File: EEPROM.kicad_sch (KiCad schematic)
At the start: 22 parts, among them IC1 PCA6408A_TSSOP, IC2 AT24CS01_SOT23, U2 TPS613221A_SOT-23-5

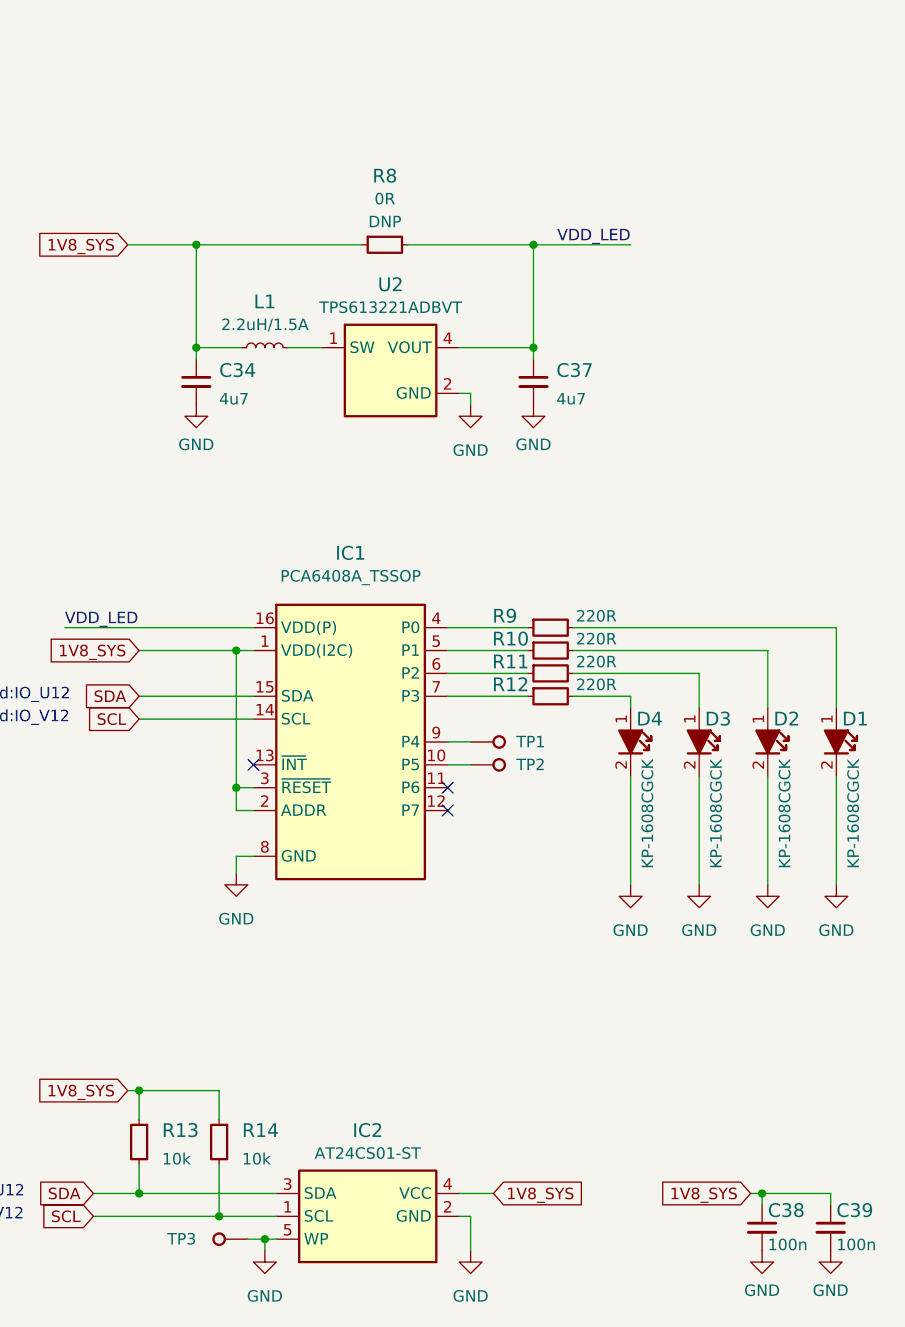
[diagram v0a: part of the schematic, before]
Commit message: Update designators
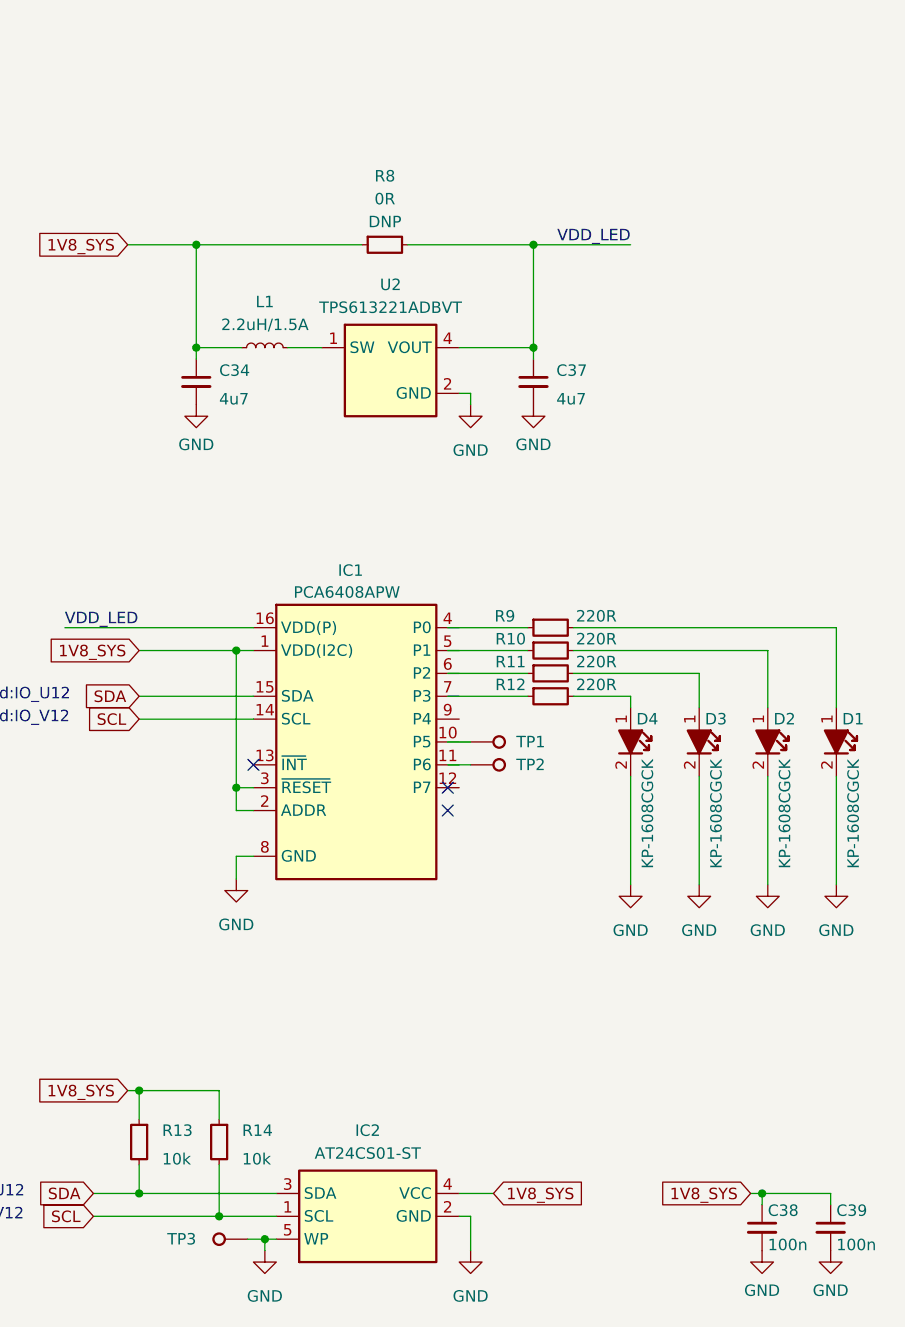
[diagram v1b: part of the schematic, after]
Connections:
- net at R9.1: no longer IC1.4 (P0)
- net at R10.1: no longer IC1.5 (P1)
- net at R11.1: no longer IC1.6 (P2)
- net at R12.1: no longer IC1.7 (P3)
- net at TP2.1: no longer IC1.10 (P5)
- net at TP1.1: no longer IC1.9 (P4)
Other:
- moved on the sheet: IC1
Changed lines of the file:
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@@
     (stroke (width 0) (type default))
   )
-  (wire (pts (xy 193.675 138.43) (xy 193.675 136.525))
+  (wire (pts (xy 193.675 139.065) (xy 193.675 136.525))
     (stroke (width 0) (type default))
   )
@@
     (in_bom yes) (on_board yes) (dnp no) (fields_autoplaced)
     (property "Reference" "C34" (at 191.77 82.5563 90)
-      (effects (font (size 1.524 1.524)) (justify left))
+      (effects (font (size 1.27 1.27)) (justify left))
     )
     (property "Value" "C_4u7_0402" (at 179.07 101.6 0)
@@
     (in_bom yes) (on_board yes) (dnp no) (fields_autoplaced)
     (property "Reference" "C37" (at 229.235 82.5563 90)
-      (effects (font (size 1.524 1.524)) (justify left))
+      (effects (font (size 1.27 1.27)) (justify left))
     )
     (property "Value" "C_4u7_0402" (at 216.535 101.6 0)
@@
     (in_bom yes) (on_board yes) (dnp no)
     (property "Reference" "IC2" (at 208.28 167.005 0)
-      (effects (font (size 1.524 1.524)))
+      (effects (font (size 1.27 1.27)))
     )
     (property "Value" "AT24CS01_SOT23" (at 208.28 168.91 0)
@@
     (in_bom yes) (on_board yes) (dnp no)
     (property "Reference" "R8" (at 210.185 60.96 0)
-      (effects (font (size 1.524 1.524)))
+      (effects (font (size 1.27 1.27)))
     )
     (property "Value" "R_0R_0402" (at 227.965 81.28 0)
@@
     (in_bom yes) (on_board yes) (dnp no) (fields_autoplaced)
     (property "Reference" "R13" (at 185.42 167.005 90)
-      (effects (font (size 1.524 1.524)) (justify left))
+      (effects (font (size 1.27 1.27)) (justify left))
     )
     (property "Value" "R_10k_0402" (at 170.18 186.055 0)
@@
     (in_bom yes) (on_board yes) (dnp no)
     (property "Reference" "R9" (at 223.52 109.855 0)
-      (effects (font (size 1.524 1.524)))
+      (effects (font (size 1.27 1.27)))
     )
     (property "Value" "R_220R_0402" (at 246.38 123.825 0)
@@
     (in_bom yes) (on_board yes) (dnp no)
     (property "Reference" "R10" (at 224.155 112.395 0)
-      (effects (font (size 1.524 1.524)))
+      (effects (font (size 1.27 1.27)))
     )
     (property "Value" "R_220R_0402" (at 246.38 126.365 0)
@@
     (in_bom yes) (on_board yes) (dnp no)
     (property "Reference" "R11" (at 224.155 114.935 0)
-      (effects (font (size 1.524 1.524)))
+      (effects (font (size 1.27 1.27)))
     )
     (property "Value" "R_220R_0402" (at 246.38 128.905 0)
@@
     (in_bom yes) (on_board yes) (dnp no)
     (property "Reference" "D4" (at 238.125 121.285 90)
-      (effects (font (size 1.524 1.524)) (justify left))
+      (effects (font (size 1.27 1.27)) (justify left))
     )
     (property "Value" "LED_G_0603_KP-1608CGCK" (at 241.3 125.7299 90)
@@
     (in_bom yes) (on_board yes) (dnp no)
     (property "Reference" "R12" (at 224.155 117.475 0)
-      (effects (font (size 1.524 1.524)))
+      (effects (font (size 1.27 1.27)))
     )
     (property "Value" "R_220R_0402" (at 246.38 131.445 0)
@@
     (in_bom yes) (on_board yes) (dnp no)
     (property "Reference" "C38" (at 252.73 175.895 90)
-      (effects (font (size 1.524 1.524)) (justify left))
+      (effects (font (size 1.27 1.27)) (justify left))
     )
     (property "Value" "C_100n_0402" (at 241.935 195.58 0)
@@
     (in_bom yes) (on_board yes) (dnp no)
     (property "Reference" "D3" (at 245.745 121.285 90)
-      (effects (font (size 1.524 1.524)) (justify left))
+      (effects (font (size 1.27 1.27)) (justify left))
     )
     (property "Value" "LED_G_0603_KP-1608CGCK" (at 248.92 125.7299 90)
@@
     (in_bom yes) (on_board yes) (dnp no)
     (property "Reference" "D2" (at 253.365 121.285 90)
-      (effects (font (size 1.524 1.524)) (justify left))
+      (effects (font (size 1.27 1.27)) (justify left))
     )
     (property "Value" "LED_G_0603_KP-1608CGCK" (at 256.54 125.7299 90)
@@
     (in_bom yes) (on_board yes) (dnp no)
     (property "Reference" "D1" (at 260.985 121.285 90)
-      (effects (font (size 1.524 1.524)) (justify left))
+      (effects (font (size 1.27 1.27)) (justify left))
     )
     (property "Value" "LED_G_0603_KP-1608CGCK" (at 264.16 125.7299 90)
@@
     )
   )
-  (symbol (lib_id "antmicropower:GND") (at 193.675 138.43 0) (unit 1)
+  (symbol (lib_id "antmicropower:GND") (at 193.675 139.065 0) (unit 1)
     (in_bom yes) (on_board yes) (dnp no) (fields_autoplaced)
-    (property "Reference" "#PWR0113" (at 193.675 144.78 0)
+    (property "Reference" "#PWR0113" (at 193.675 145.415 0)
       (effects (font (size 1.27 1.27)) hide)
     )
-    (property "Value" "GND" (at 193.675 143.51 0)
+    (property "Value" "GND" (at 193.675 144.145 0)
       (effects (font (size 1.27 1.27)))
     )
-    (property "Footprint" "" (at 193.675 138.43 0)
+    (property "Footprint" "" (at 193.675 139.065 0)
       (effects (font (size 1.27 1.27)) hide)
     )
-    (property "Datasheet" "" (at 193.675 138.43 0)
+    (property "Datasheet" "" (at 193.675 139.065 0)
       (effects (font (size 1.27 1.27)) hide)
     )
@@
     (in_bom yes) (on_board yes) (dnp no)
     (property "Reference" "L1" (at 196.85 74.93 0)
-      (effects (font (size 1.524 1.524)))
+      (effects (font (size 1.27 1.27)))
     )
     (property "Value" "L_2.2u_1.5A_0806" (at 208.28 82.55 0)
@@
     (in_bom yes) (on_board yes) (dnp no)
     (property "Reference" "U2" (at 210.82 73.025 0)
-      (effects (font (size 1.524 1.524)))
+      (effects (font (size 1.27 1.27)))
     )
     (property "Value" "TPS613221A_SOT-23-5" (at 210.82 74.93 0)
@@
     (in_bom yes) (on_board yes) (dnp no) (fields_autoplaced)
     (property "Reference" "R14" (at 194.31 167.005 90)
-      (effects (font (size 1.524 1.524)) (justify left))
+      (effects (font (size 1.27 1.27)) (justify left))
     )
     (property "Value" "R_10k_0402" (at 179.07 186.055 0)
@@
     (in_bom yes) (on_board yes) (dnp no)
     (property "Reference" "C39" (at 260.35 175.895 90)
-      (effects (font (size 1.524 1.524)) (justify left))
+      (effects (font (size 1.27 1.27)) (justify left))
     )
     (property "Value" "C_100n_0402" (at 249.555 195.58 0)
@@
   )
   (symbol (lib_id "antmicroInterfaceIOExpanders:PCA6408A_TSSOP") (at 195.58 111.125 0) (unit 1)
-    (in_bom yes) (on_board yes) (dnp no) (fields_autoplaced)
-    (property "Reference" "IC1" (at 206.375 102.87 0)
-      (effects (font (size 1.524 1.524)))
+    (in_bom yes) (on_board yes) (dnp no)
+    (property "Reference" "IC1" (at 206.375 104.775 0)
+      (effects (font (size 1.27 1.27)))
     )
     (property "Value" "PCA6408A_TSSOP" (at 206.375 105.41 0)
-      (effects (font (size 1.27 1.27) (thickness 0.15)))
+      (effects (font (size 1.27 1.27) (thickness 0.15)) hide)
     )
     (property "Footprint" "antmicro-footprints:TSSOP-16_4.4x5mm_P0.65mm" (at 231.14 118.745 0)
       (effects (font (size 1.27 1.27) (thickness 0.15)) (justify left bottom) hide)
     )
-    (property "Datasheet" "https://www.mouser.pl/datasheet/2/302/PCA6408A-1127604.pdf" (at 231.14 121.285 0)
+    (property "Datasheet" "https://www.mouser.com/datasheet/2/302/PCA6408A-1127604.pdf" (at 231.14 121.285 0)
       (effects (font (size 1.27 1.27) (thickness 0.15)) (justify left bottom) hide)
     )
@@
       (effects (font (size 1.27 1.27) (thickness 0.15)) (justify left bottom) hide)
     )
-    (property "MPN" "PCA6408APW" (at 231.14 126.365 0)
-      (effects (font (size 1.27 1.27) (thickness 0.15)) (justify left bottom) hide)
+    (property "MPN" "PCA6408APW" (at 200.025 107.95 0)
+      (effects (font (size 1.27 1.27) (thickness 0.15)) (justify left bottom))
     )
     (property "Author" "Antmicro" (at 231.14 128.905 0)
